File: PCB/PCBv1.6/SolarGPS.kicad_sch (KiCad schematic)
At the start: 46 parts, among them J1 Conn_01x10_Female, J2 Solar2+, J3 Solar1+, J4 GND, J5 GND, J6 Conn_02x03_Odd_Even, J7 Screw_Terminal_01x01, J8 Conn_01x04_Male, U1 BQ25505, U2 MAX-M10Q, U3 STM32L031G6Ux, U4 MAX40200AUK, U6 LIS3DH, Y1 32.768

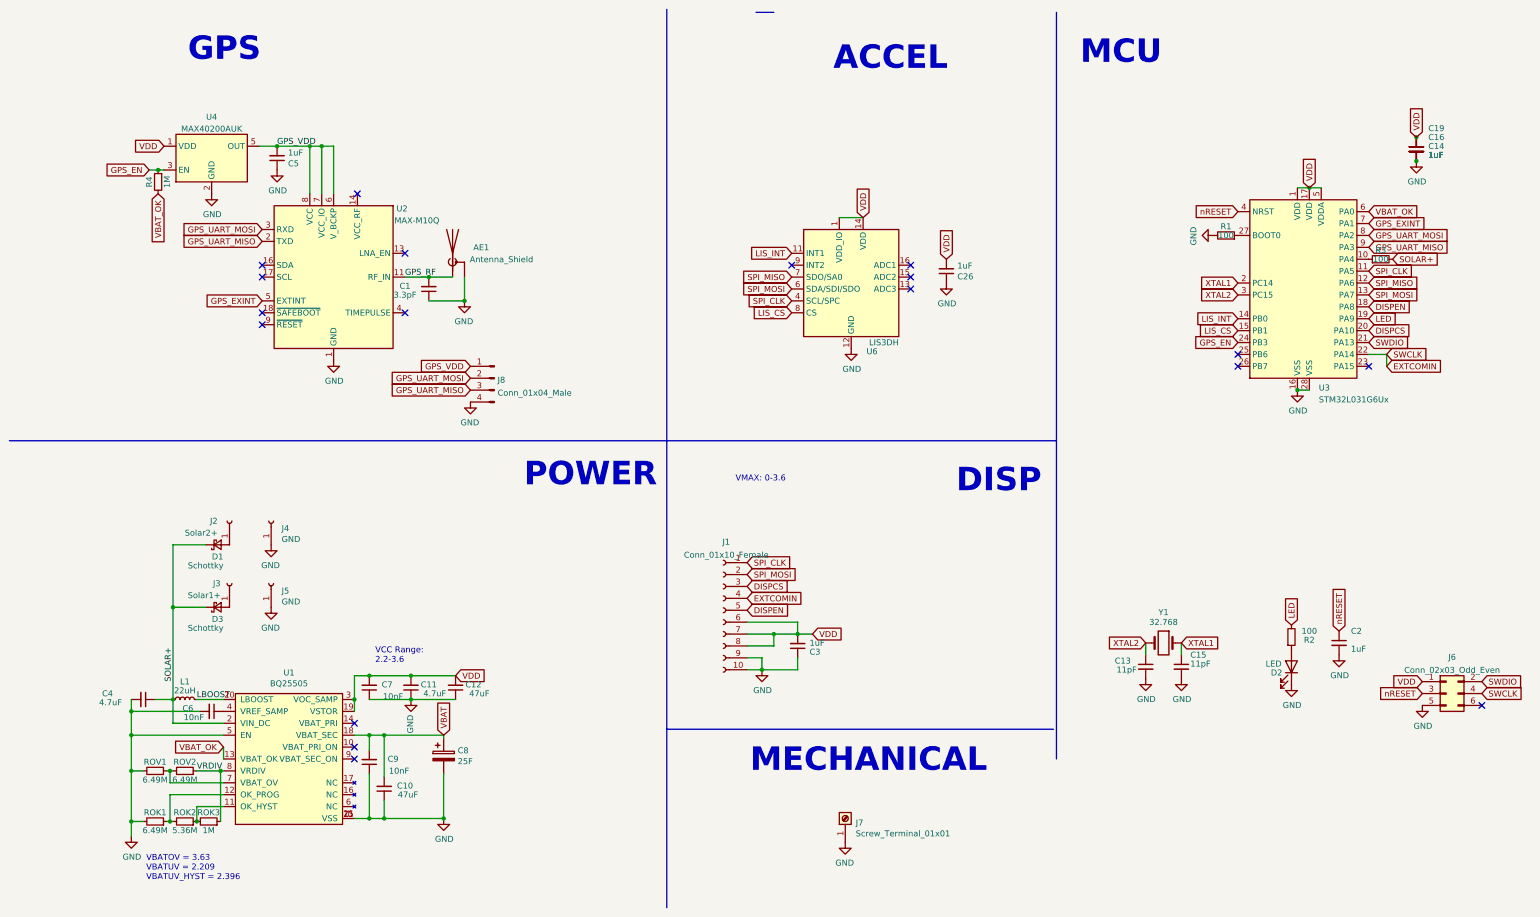
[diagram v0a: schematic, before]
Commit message: More Progress
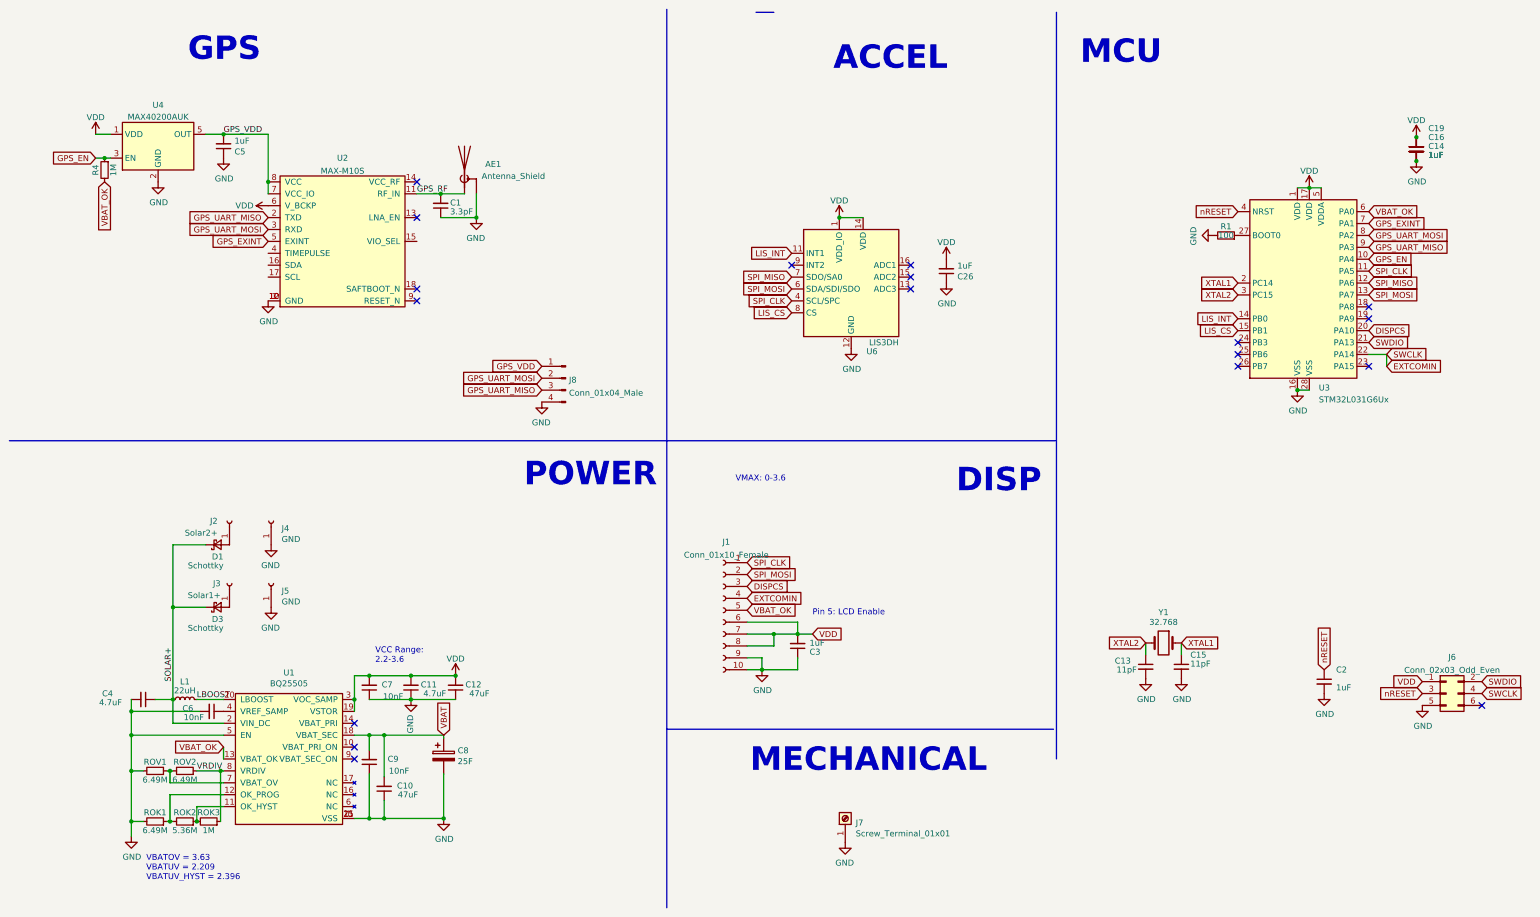
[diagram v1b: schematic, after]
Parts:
- removed D2: LED, Diode_SMD:D_0805_2012Metric, symbol Device:LED
- removed R2, R3: 100, Resistor_SMD:R_0603_1608Metric, symbol Device:R_Small
- removed U2: MAX-M10Q, RF_GPS:ublox_MAX, symbol RF_GPS:MAX-M8Q
- added U2: MAX-M10S, Margo_Lib:MAX-8, symbol MargoGeneral:MAX-M10S
- C8: symbol Device:CP -> Device:C_Polarized
- U1: footprint Package_DFN_QFN:QFN-20-1EP_3.5x3.5mm_P0.5mm_EP2x2mm -> Package_DFN_QFN:Texas_VQFN-RGR-20
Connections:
- net GND: now also U2.1 (GND), U2.10 (GND), U2.12 (GND)
- net GPS_EN: now also U3.10 (PA4); no longer U3.24 (PB3)
- net GPS_EXINT: now also U2.5 (EXINT)
- net GPS_RF: now also U2.11 (RF_IN)
- net GPS_UART_MISO: now also U2.2 (TXD)
- net GPS_UART_MOSI: now also U2.3 (RXD)
- net GPS_VDD: now also U2.7 (VCC_IO), U2.8 (VCC)
- net VBAT_OK: now also J1.5 (Pin_5)
- net VDD: now also U2.6 (V_BCKP)
- net DISPEN: no longer names the net of U3.18 (PA8)
- net DISPEN: no longer J1.5 (Pin_5)
- net LED: no longer names the net of U3.19 (PA9)
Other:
- note added: "Pin 5: LCD Enable"
- moved on the sheet: AE1, C1, C2, C5, J8, R4, U4
